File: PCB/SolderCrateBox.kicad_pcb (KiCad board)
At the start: 4 copper layers, 100 x 40 mm, 60 parts, among them IC1 MC34063ADR, IC2 ESP32-C3-MINI-1U-N4X, J1 Conn_01x02, J2 Conn_01x02, J3 Conn_01x03, J4 Conn_01x03, J5 USB_C_Receptacle_USB2.0_16P, Q1 BSS84, Q2 2N7002, SW10 SW_Push, SW11 SW_Push, U1 AMS1117-3.3, U2 USBLC6-2SC6

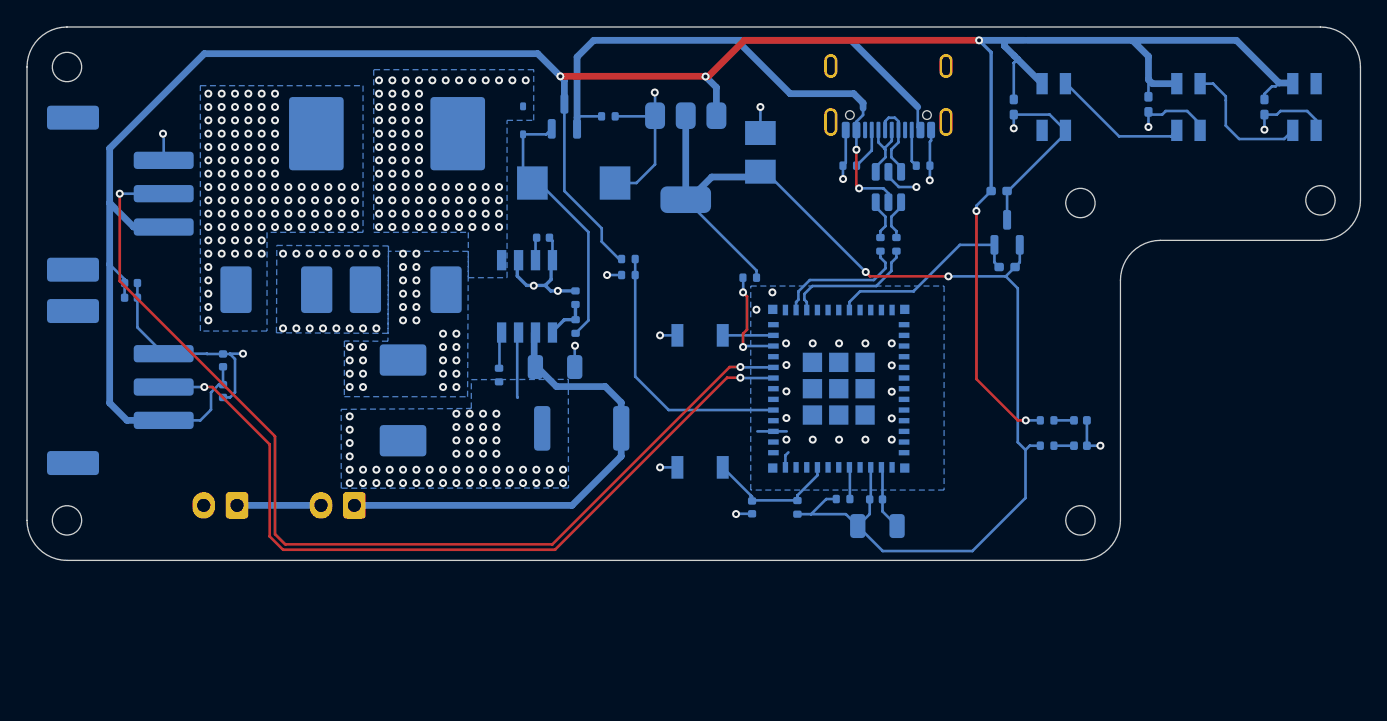
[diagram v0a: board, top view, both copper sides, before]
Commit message: Initial Commit for INA219
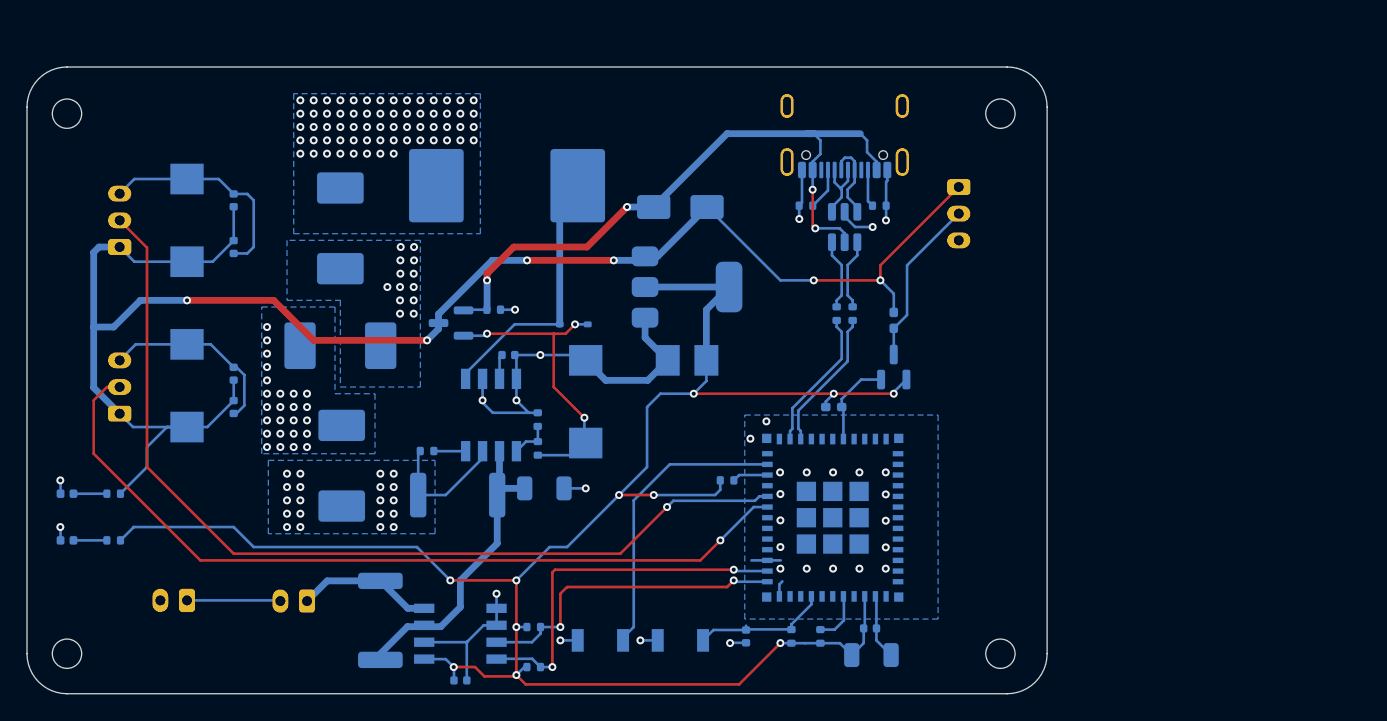
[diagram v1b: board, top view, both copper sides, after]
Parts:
- removed C12, C13, C14: 100n, Capacitor_SMD:C_0402_1005Metric_Pad0.74x0.62mm_HandSolder
- removed D7, D8, D9: WS2812B, LED_SMD:LED_SK6812MINI_PLCC4_3.5x3.5mm_P1.75mm
- removed R27: 5.1k, Resistor_SMD:R_0402_1005Metric
- removed R28: 10k, Resistor_SMD:R_0402_1005Metric
- removed the REF** at (210.0, 51.2)
- added C11: TAJE477K010RNJ, Footprints:CAPPM7344X430N, B.Cu at (143.0, 52.5)
- added C17: 100n, Capacitor_SMD:C_0402_1005Metric, B.Cu at (163.5, 87.0)
- added C9: TAJE477K010RNJ, Footprints:CAPPM7344X430N, B.Cu at (143.0, 64.9)
- added D2: SS12, Diode_SMD:D_SMA, B.Cu at (180.0, 51.5)
- added IC5: INA219AIDR, Footprints:SOIC127P600X175-8N, B.Cu at (163.5, 83.5)
- added J6: Conn_01x03, Connector_JST:JST_PH_S3B-PH-K_1x03_P2.00mm_Horizontal, B.Cu at (200.9, 50.0)
- added R11: 0.01, Resistor_SMD:R_2512_6332Metric, B.Cu at (157.5, 82.5)
- added R8: 10K, Resistor_SMD:R_0402_1005Metric, B.Cu at (169.0, 86.0)
- added R9: 10K, Resistor_SMD:R_0402_1005Metric, B.Cu at (169.0, 83.0)
- J1, J2: footprint Connector_JST:JST_XH_B2B-XH-A_1x02_P2.50mm_Vertical -> Connector_JST:JST_PH_S2B-PH-K_1x02_P2.00mm_Horizontal
- J3, J4: footprint Connector_JST:JST_XH_S3B-XH-SM4-TB_1x03-1MP_P2.50mm_Horizontal -> Connector_JST:JST_PH_S3B-PH-K_1x03_P2.00mm_Horizontal
- R3: value 3k3 -> 10k
- R4: value 10k -> 39k
- moved D20 76.3 mm to (134.0, 76.5), turned to 0 degrees
- moved D19 76.2 mm to (134.0, 73.0), turned to 0 degrees
- moved R22 70.4 mm to (137.5, 76.5), turned to 0 degrees
- moved R21 70.2 mm to (137.5, 73.0), turned to 0 degrees
- moved REF** 24.9 mm to (204.0, 44.5)
- moved SW11 24.1 mm to (174.0, 84.0)
- moved Q1 17.7 mm to (162.8, 60.2), turned to 180 degrees
- moved R5 16.9 mm to (166.0, 59.2)
- moved R13 16.7 mm to (191.5, 66.5), turned to 0 degrees
- moved C8 16.5 mm to (180.5, 63.0), turned to 180 degrees
- moved J3 16.5 mm to (137.9, 67.0)
- moved C6 16.4 mm to (172.9, 66.1), turned to 90 degrees
- moved D1 15.8 mm to (172.0, 60.3), turned to 180 degrees
- moved R23 15.3 mm to (183.5, 72.0), turned to 0 degrees
- moved Q2 13.2 mm to (196.0, 63.5)
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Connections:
- net +V_{BATT} renamed +V_{SYS}
- net /ESP32/BOOT renamed /ESP32_C3/BOOT
- net /ESP32/D+ renamed /ESP32_C3/D+
- net /ESP32/D- renamed /ESP32_C3/D-
- net /ESP32/DR+ renamed /ESP32_C3/DR+
- net /ESP32/DR- renamed /ESP32_C3/DR-
- net /ESP32/GPIO2 renamed /ESP32_C3/GPIO2
- net /ESP32/GPIO20 renamed /ESP32_C3/GPIO20
- net /ESP32/GPIO3 renamed /ESP32_C3/GPIO3
- net /ESP32/GPIO4 renamed /ESP32_C3/GPIO4
- net /ESP32/GPIO7 renamed /ESP32_C3/GPIO7
- net /ESP32/GPIO8 renamed /ESP32_C3/GPIO8
- net /ESP32/RST renamed /ESP32_C3/RST
- net /ESP32/USB_D+ renamed /ESP32_C3/USB_D+
- net /ESP32/USB_D- renamed /ESP32_C3/USB_D-
- C5 pad 1: /Boost/BATT_{IN} -> /VI_Sensor/IN-
- IC1 pad 6: /Boost/BATT_{IN} -> /VI_Sensor/IN-
- IC2 pad 12: /ESP32/GPIO0 -> /I2C.SDA
- IC2 pad 13: /ESP32/GPIO1 -> /I2C.SCL
- IC2 pad 16: /Boost/V_{Sense} -> /ESP32_C3/GPIO10
- IC2 pad 19: /PWM.SRV2 -> /PWM.SRV1
- IC2 pad 20: /PWM.SRV1 -> /PWM.SRV2
- J2 pad 1: /Boost/BATT_{IN} -> /VI_Sensor/IN+
- R1 pad 1: /Boost/BATT_{IN} -> /VI_Sensor/IN-
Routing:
- net +V_{SYS}: track 202.6 -> 126.9 mm, vias 5 -> 6
- net +3V3: track 90.6 -> 144.4 mm, vias 2 -> 11
- net /Boost/BATT_{IN}: track 35.6 -> 0.00 mm
- net /I2C.SCL: track 0.00 -> 27.8 mm, vias 0 -> 2
- net /I2C.SDA: track 0.00 -> 24.0 mm, vias 0 -> 2
- net /VI_Sensor/IN-: track 0.00 -> 22.4 mm
- net /Boost/V_{Sense}: track 20.2 -> 0.00 mm
- net Net-(D1-A): track 0.00 -> 19.9 mm, vias 80 -> 0
- net /ESP32_C3/BOOT: track 3.70 -> 22.0 mm
- net /PWM.SRV1: track 76.9 -> 61.9 mm, vias 2 -> 1
- net Net-(D8-DOUT): track 10.4 -> 0.00 mm
- net /PWM.SRV2: track 60.1 -> 70.3 mm, vias 2 -> 1
- net Net-(D7-DOUT): track 10.1 -> 0.00 mm
- net /VI_Sensor/IN+: track 0.00 -> 9.77 mm
- net GND: track 88.1 -> 96.9 mm, vias 36 -> 32
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- removed copper zone on B.Cu, net Net-(D1-A)
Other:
- board size 100 x 40 mm -> 76.5 x 47 mm
- board text added: "LED"
- board text added: "SRV1"
- board text added: "SRV2"
- board text added: "SW_Solder V2.0"
- board text added: "V_{SYS}"
- board text removed: "SW_Solder V1.1"
- board text removed: "V_{BATT}"
